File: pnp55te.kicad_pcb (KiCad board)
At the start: 2 copper layers, 154 x 109 mm, 68 parts, among them P1 1123038-2, U1 VNLD5090, U2 VNLD5090, U3 molex_48pin_MRE, U4 ITEAD_HC-05

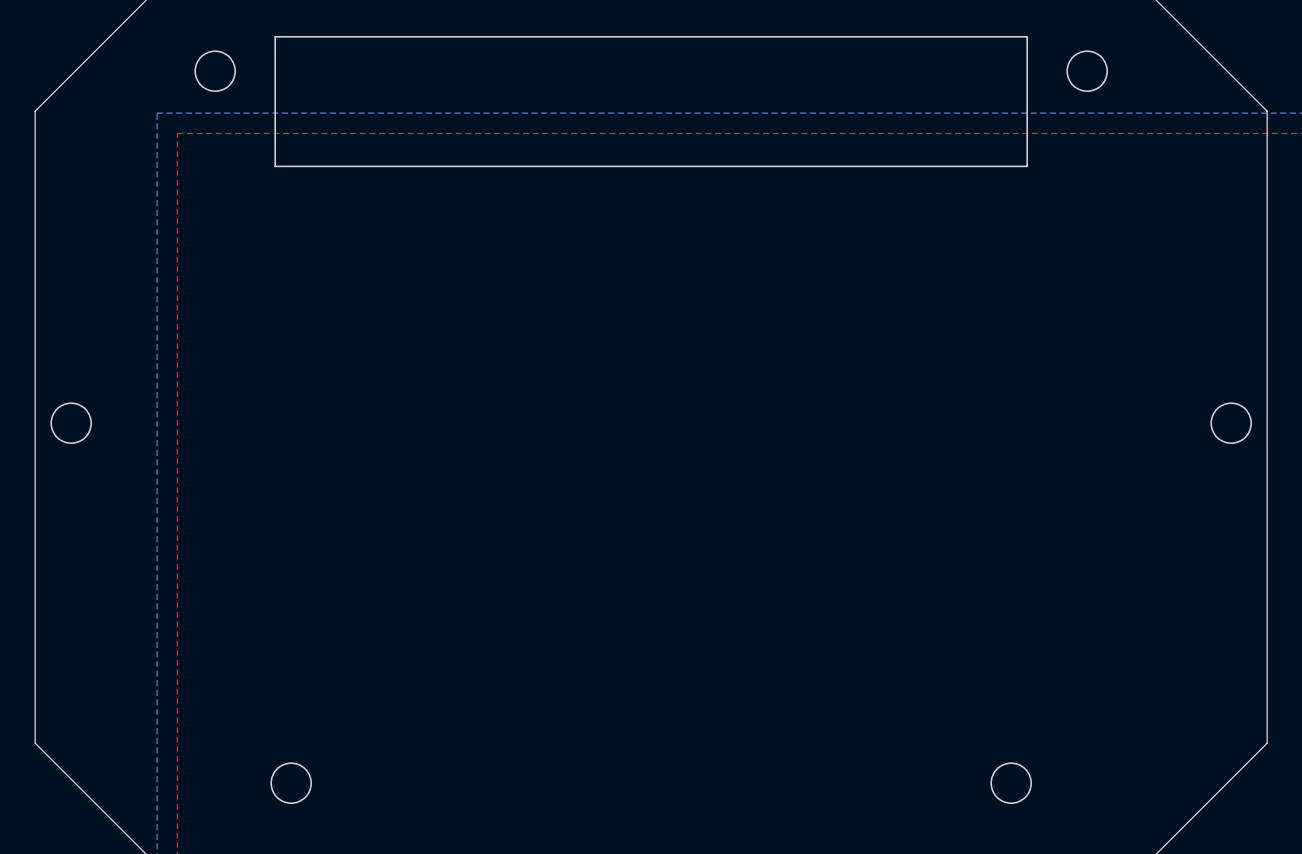
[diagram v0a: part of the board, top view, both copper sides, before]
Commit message: progress
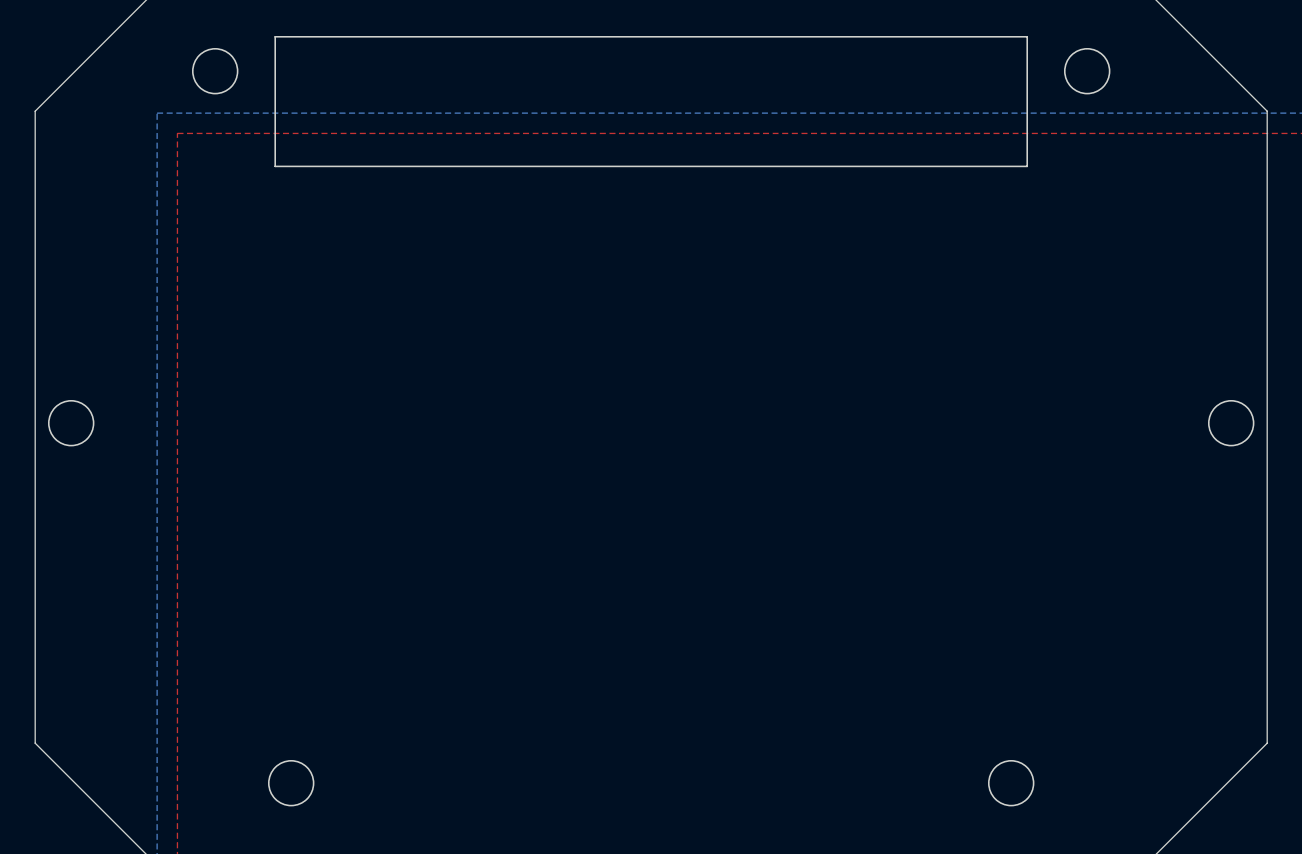
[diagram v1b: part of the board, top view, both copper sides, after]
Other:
- outline, holes or cut-outs redrawn
- board text added: "Vertical clearance: (including PCB material) 8.3mm total on sides 10.3 (2mm extra) in the middle"
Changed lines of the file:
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@@
   (general
     (thickness 1.6)
-    (drawings 25)
+    (drawings 26)
     (tracks 0)
     (zones 0)
@@
     )
   )
+  (gr_text "Vertical clearance:\n(including PCB material)\n8.3mm total on sides\n10.3 (2mm extra) in the middle" (at -28.6 -18.8) (layer Cmts.User)
+    (effects (font (size 4 4) (thickness 0.15)))
+  )
   (gr_line (start 124 5.7) (end 30 5.7) (layer Edge.Cuts) (width 0.2))
   (gr_line (start 124 21.9) (end 124 5.7) (layer Edge.Cuts) (width 0.2))
   (gr_line (start 30 21.9) (end 124 21.9) (layer Edge.Cuts) (width 0.2))
   (gr_line (start 30 5.7) (end 30 21.9) (layer Edge.Cuts) (width 0.2))
-  (gr_circle (center 131.5 10) (end 134 10) (layer Edge.Cuts) (width 0.2))
+  (gr_circle (center 131.5 10) (end 134.3 10) (layer Edge.Cuts) (width 0.2))
   (gr_line (start 0 94) (end 15 109) (layer Edge.Cuts) (width 0.1))
   (gr_line (start 139 109) (end 154 94) (layer Edge.Cuts) (width 0.1))
@@
     (effects (font (size 1.5 1.5) (thickness 0.3)))
   )
-  (gr_circle (center 32 99) (end 34.5 99) (layer Edge.Cuts) (width 0.2))
-  (gr_circle (center 122 99) (end 124.5 99) (layer Edge.Cuts) (width 0.2))
-  (gr_circle (center 149.5 54) (end 152 54) (layer Edge.Cuts) (width 0.2))
-  (gr_circle (center 22.5 10) (end 25 10) (layer Edge.Cuts) (width 0.2))
-  (gr_circle (center 4.5 54) (end 7 54) (layer Edge.Cuts) (width 0.2))
+  (gr_circle (center 32 99) (end 34.8 99) (layer Edge.Cuts) (width 0.2))
+  (gr_circle (center 122 99) (end 124.8 99) (layer Edge.Cuts) (width 0.2))
+  (gr_circle (center 149.5 54) (end 152.3 54) (layer Edge.Cuts) (width 0.2))
+  (gr_circle (center 22.5 10) (end 25.3 10) (layer Edge.Cuts) (width 0.2))
+  (gr_circle (center 4.5 54) (end 7.3 54) (layer Edge.Cuts) (width 0.2))
   (gr_line (start 15 0) (end 139 0) (layer Edge.Cuts) (width 0.1))
   (gr_line (start 154 15) (end 154 94) (layer Edge.Cuts) (width 0.1))
